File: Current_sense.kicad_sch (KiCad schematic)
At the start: 12 parts, among them U33 INA180A4

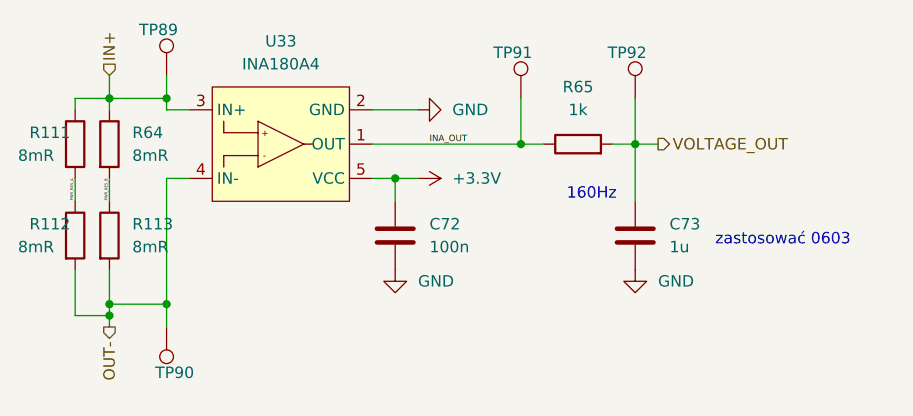
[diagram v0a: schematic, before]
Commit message: v2.1 finished
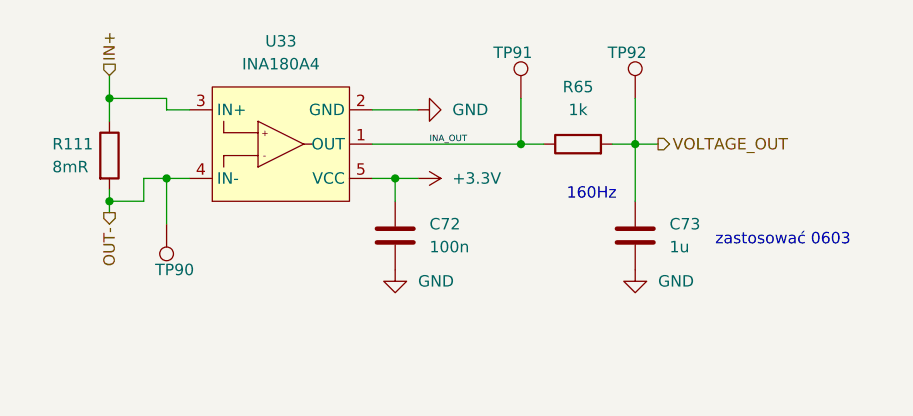
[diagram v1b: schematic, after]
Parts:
- removed R112, R113, R64: 8mR, Resistor_SMD:R_2512_6332Metric_Pad1.40x3.35mm_HandSolder, symbol Device:R
- removed TP89: TestPoint, TestPoint:TestPoint_THTPad_1.0x1.0mm_Drill0.5mm, symbol Connector:TestPoint
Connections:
- net PWR_RES_A is gone; now on net OUT-: R111.2
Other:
- moved on the sheet: R111, TP90
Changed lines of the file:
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@@
   (junction (at 104.14 77.47) (diameter 0) (color 0 0 0 0)
   )
-  (junction (at 110.49 77.47) (diameter 0) (color 0 0 0 0)
-  )
-  (junction (at 110.49 100.33) (diameter 0) (color 0 0 0 0)
-  )
-  (junction (at 104.14 100.33) (diameter 0) (color 0 0 0 0)
-  )
-  (junction (at 104.14 101.6) (diameter 0) (color 0 0 0 0)
+  (junction (at 104.14 88.9) (diameter 0) (color 0 0 0 0)
+  )
+  (junction (at 110.49 86.36) (diameter 0) (color 0 0 0 0)
   )
   (wire (pts (xy 110.49 77.47) (xy 110.49 78.74))
@@
     (stroke (width 0) (type default) (color 0 0 0 0))
   )
-  (wire (pts (xy 104.14 96.52) (xy 104.14 100.33))
-    (stroke (width 0) (type default) (color 0 0 0 0))
-  )
-  (wire (pts (xy 104.14 78.74) (xy 104.14 77.47))
+  (wire (pts (xy 104.14 88.9) (xy 104.14 90.17))
+    (stroke (width 0) (type default) (color 0 0 0 0))
+  )
+  (wire (pts (xy 104.14 77.47) (xy 104.14 80.01))
+    (stroke (width 0) (type default) (color 0 0 0 0))
+  )
+  (wire (pts (xy 107.95 88.9) (xy 107.95 86.36))
+    (stroke (width 0) (type default) (color 0 0 0 0))
+  )
+  (wire (pts (xy 104.14 88.9) (xy 107.95 88.9))
     (stroke (width 0) (type default) (color 0 0 0 0))
   )
@@
     (stroke (width 0) (type default) (color 0 0 0 0))
   )
-  (wire (pts (xy 110.49 100.33) (xy 110.49 102.87))
-    (stroke (width 0) (type default) (color 0 0 0 0))
-  )
   (wire (pts (xy 135.89 86.36) (xy 135.89 88.9))
     (stroke (width 0) (type default) (color 0 0 0 0))
   )
-  (wire (pts (xy 110.49 100.33) (xy 104.14 100.33))
-    (stroke (width 0) (type default) (color 0 0 0 0))
-  )
-  (wire (pts (xy 104.14 88.9) (xy 104.14 86.36))
-    (stroke (width 0) (type default) (color 0 0 0 0))
-  )
-  (wire (pts (xy 100.33 77.47) (xy 104.14 77.47))
-    (stroke (width 0) (type default) (color 0 0 0 0))
-  )
   (wire (pts (xy 104.14 74.93) (xy 104.14 77.47))
     (stroke (width 0) (type default) (color 0 0 0 0))
   )
-  (wire (pts (xy 110.49 86.36) (xy 110.49 100.33))
-    (stroke (width 0) (type default) (color 0 0 0 0))
-  )
-  (wire (pts (xy 104.14 101.6) (xy 104.14 102.87))
-    (stroke (width 0) (type default) (color 0 0 0 0))
-  )
-  (wire (pts (xy 110.49 74.93) (xy 110.49 77.47))
-    (stroke (width 0) (type default) (color 0 0 0 0))
-  )
-  (wire (pts (xy 100.33 101.6) (xy 104.14 101.6))
-    (stroke (width 0) (type default) (color 0 0 0 0))
-  )
-  (wire (pts (xy 100.33 78.74) (xy 100.33 77.47))
+  (wire (pts (xy 110.49 86.36) (xy 113.03 86.36))
+    (stroke (width 0) (type default) (color 0 0 0 0))
+  )
+  (wire (pts (xy 104.14 87.63) (xy 104.14 88.9))
+    (stroke (width 0) (type default) (color 0 0 0 0))
+  )
+  (wire (pts (xy 110.49 86.36) (xy 110.49 91.44))
     (stroke (width 0) (type default) (color 0 0 0 0))
   )
@@
     (stroke (width 0) (type default) (color 0 0 0 0))
   )
-  (wire (pts (xy 113.03 86.36) (xy 110.49 86.36))
+  (wire (pts (xy 107.95 86.36) (xy 110.49 86.36))
     (stroke (width 0) (type default) (color 0 0 0 0))
   )
@@
     (stroke (width 0) (type default) (color 0 0 0 0))
   )
-  (wire (pts (xy 104.14 100.33) (xy 104.14 101.6))
-    (stroke (width 0) (type default) (color 0 0 0 0))
-  )
   (wire (pts (xy 133.35 82.55) (xy 149.86 82.55))
     (stroke (width 0) (type default) (color 0 0 0 0))
@@
     (stroke (width 0) (type default) (color 0 0 0 0))
   )
-  (wire (pts (xy 100.33 96.52) (xy 100.33 101.6))
-    (stroke (width 0) (type default) (color 0 0 0 0))
-  )
   (wire (pts (xy 104.14 77.47) (xy 110.49 77.47))
     (stroke (width 0) (type default) (color 0 0 0 0))
@@
   )
   (wire (pts (xy 135.89 86.36) (xy 133.35 86.36))
-    (stroke (width 0) (type default) (color 0 0 0 0))
-  )
-  (wire (pts (xy 100.33 88.9) (xy 100.33 86.36))
     (stroke (width 0) (type default) (color 0 0 0 0))
   )
@@
     (effects (font (size 1.27 1.27)) (justify left bottom))
   )
-  (label "PWR_RES_B" (at 104.14 86.36 270)
-    (effects (font (size 0.3 0.3)) (justify right bottom))
-  )
   (label "INA_OUT" (at 139.7 82.55 0)
     (effects (font (size 0.7 0.7)) (justify left bottom))
   )
-  (label "PWR_RES_A" (at 100.33 86.36 270)
-    (effects (font (size 0.3 0.3)) (justify right bottom))
-  )
-  (hierarchical_label "OUT-" (shape output) (at 104.14 102.87 270)
+  (hierarchical_label "OUT-" (shape output) (at 104.14 90.17 270)
     (effects (font (size 1.27 1.27)) (justify right))
   )
@@
     (pin "1")
   )
-  (symbol (lib_id "Device:R") (at 100.33 92.71 0) (unit 1)
-    (in_bom yes) (on_board yes)
-    (property "Reference" "R112" (id 0) (at 95.25 91.44 0)
-      (effects (font (size 1.27 1.27)) (justify left))
-    )
-    (property "Value" "8mR" (id 1) (at 93.98 93.98 0)
-      (effects (font (size 1.27 1.27)) (justify left))
-    )
-    (property "Footprint" "Resistor_SMD:R_2512_6332Metric_Pad1.40x3.35mm_HandSolder" (id 2) (at 98.552 92.71 90)
-      (effects (font (size 1.27 1.27)) hide)
-    )
-    (property "Datasheet" "~" (id 3) (at 100.33 92.71 0)
-      (effects (font (size 1.27 1.27)) hide)
-    )
-    (pin "1")
-    (pin "2")
-  )
-  (symbol (lib_id "Connector:TestPoint") (at 110.49 74.93 0) (unit 1)
-    (in_bom yes) (on_board yes)
-    (property "Reference" "TP89" (id 0) (at 111.76 69.85 0)
-      (effects (font (size 1.27 1.27)) (justify right))
-    )
-    (property "Value" "TestPoint" (id 1) (at 107.95 70.3581 0)
-      (effects (font (size 1.27 1.27)) (justify right) hide)
-    )
-    (property "Footprint" "TestPoint:TestPoint_THTPad_1.0x1.0mm_Drill0.5mm" (id 2) (at 115.57 74.93 0)
-      (effects (font (size 1.27 1.27)) hide)
-    )
-    (property "Datasheet" "~" (id 3) (at 115.57 74.93 0)
-      (effects (font (size 1.27 1.27)) hide)
-    )
-    (pin "1")
-  )
   (symbol (lib_id "_IntegratedCircuits:INA180A4") (at 123.19 82.55 0) (mirror x) (unit 1)
     (in_bom yes) (on_board yes) (fields_autoplaced)
@@
     (pin "1")
   )
-  (symbol (lib_id "Device:R") (at 104.14 82.55 0) (unit 1)
-    (in_bom yes) (on_board yes) (fields_autoplaced)
-    (property "Reference" "R64" (id 0) (at 106.68 81.2799 0)
-      (effects (font (size 1.27 1.27)) (justify left))
-    )
-    (property "Value" "8mR" (id 1) (at 106.68 83.8199 0)
-      (effects (font (size 1.27 1.27)) (justify left))
-    )
-    (property "Footprint" "Resistor_SMD:R_2512_6332Metric_Pad1.40x3.35mm_HandSolder" (id 2) (at 102.362 82.55 90)
-      (effects (font (size 1.27 1.27)) hide)
-    )
-    (property "Datasheet" "~" (id 3) (at 104.14 82.55 0)
-      (effects (font (size 1.27 1.27)) hide)
-    )
-    (pin "1")
-    (pin "2")
-  )
   (symbol (lib_id "power:GND") (at 162.56 96.52 0) (unit 1)
     (in_bom yes) (on_board yes) (fields_autoplaced)
@@
     )
     (pin "1")
-  )
-  (symbol (lib_id "Device:R") (at 104.14 92.71 0) (unit 1)
-    (in_bom yes) (on_board yes) (fields_autoplaced)
-    (property "Reference" "R113" (id 0) (at 106.68 91.4399 0)
-      (effects (font (size 1.27 1.27)) (justify left))
-    )
-    (property "Value" "8mR" (id 1) (at 106.68 93.9799 0)
-      (effects (font (size 1.27 1.27)) (justify left))
-    )
-    (property "Footprint" "Resistor_SMD:R_2512_6332Metric_Pad1.40x3.35mm_HandSolder" (id 2) (at 102.362 92.71 90)
-      (effects (font (size 1.27 1.27)) hide)
-    )
-    (property "Datasheet" "~" (id 3) (at 104.14 92.71 0)
-      (effects (font (size 1.27 1.27)) hide)
-    )
-    (pin "1")
-    (pin "2")
   )
   (symbol (lib_id "Device:R") (at 156.21 82.55 90) (unit 1)
@@
     (pin "1")
   )
-  (symbol (lib_id "Device:R") (at 100.33 82.55 0) (unit 1)
+  (symbol (lib_id "Device:R") (at 104.14 83.82 0) (unit 1)
     (in_bom yes) (on_board yes)
-    (property "Reference" "R111" (id 0) (at 95.25 81.28 0)
-      (effects (font (size 1.27 1.27)) (justify left))
-    )
-    (property "Value" "8mR" (id 1) (at 93.98 83.82 0)
-      (effects (font (size 1.27 1.27)) (justify left))
-    )
-    (property "Footprint" "Resistor_SMD:R_2512_6332Metric_Pad1.40x3.35mm_HandSolder" (id 2) (at 98.552 82.55 90)
-      (effects (font (size 1.27 1.27)) hide)
-    )
-    (property "Datasheet" "~" (id 3) (at 100.33 82.55 0)
+    (property "Reference" "R111" (id 0) (at 97.79 82.55 0)
+      (effects (font (size 1.27 1.27)) (justify left))
+    )
+    (property "Value" "8mR" (id 1) (at 97.79 85.09 0)
+      (effects (font (size 1.27 1.27)) (justify left))
+    )
+    (property "Footprint" "Resistor_SMD:R_2512_6332Metric_Pad1.40x3.35mm_HandSolder" (id 2) (at 102.362 83.82 90)
+      (effects (font (size 1.27 1.27)) hide)
+    )
+    (property "Datasheet" "~" (id 3) (at 104.14 83.82 0)
       (effects (font (size 1.27 1.27)) hide)
     )
@@
     (pin "2")
   )
-  (symbol (lib_id "Connector:TestPoint") (at 110.49 102.87 180) (unit 1)
+  (symbol (lib_id "Connector:TestPoint") (at 110.49 91.44 180) (unit 1)
     (in_bom yes) (on_board yes)
-    (property "Reference" "TP90" (id 0) (at 109.22 107.95 0)
+    (property "Reference" "TP90" (id 0) (at 109.22 96.52 0)
       (effects (font (size 1.27 1.27)) (justify right))
     )
-    (property "Value" "TestPoint" (id 1) (at 113.03 107.4419 0)
+    (property "Value" "TestPoint" (id 1) (at 113.03 96.0119 0)
       (effects (font (size 1.27 1.27)) (justify right) hide)
     )
-    (property "Footprint" "TestPoint:TestPoint_THTPad_1.0x1.0mm_Drill0.5mm" (id 2) (at 105.41 102.87 0)
-      (effects (font (size 1.27 1.27)) hide)
-    )
-    (property "Datasheet" "~" (id 3) (at 105.41 102.87 0)
-      (effects (font (size 1.27 1.27)) hide)
-    )
+    (property "Footprint" "TestPoint:TestPoint_THTPad_1.0x1.0mm_Drill0.5mm" (id 2) (at 105.41 91.44 0)
+      (effects (font (size 1.27 1.27)) hide)
+    )
+    (property "Datasheet" "~" (id 3) (at 105.41 91.44 0)
+      (effects (font (size 1.27 1.27)) hide)
+    )
